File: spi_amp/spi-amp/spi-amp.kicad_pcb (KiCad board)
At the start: 4 copper layers, 26.9 x 54.8 mm, 25 parts, among them J1 IN+, J2 IN-, J3 OUT+, J4 OUT-, J5 Conn_01x06, U1 LMH6401, U2 LM78M05_TO220

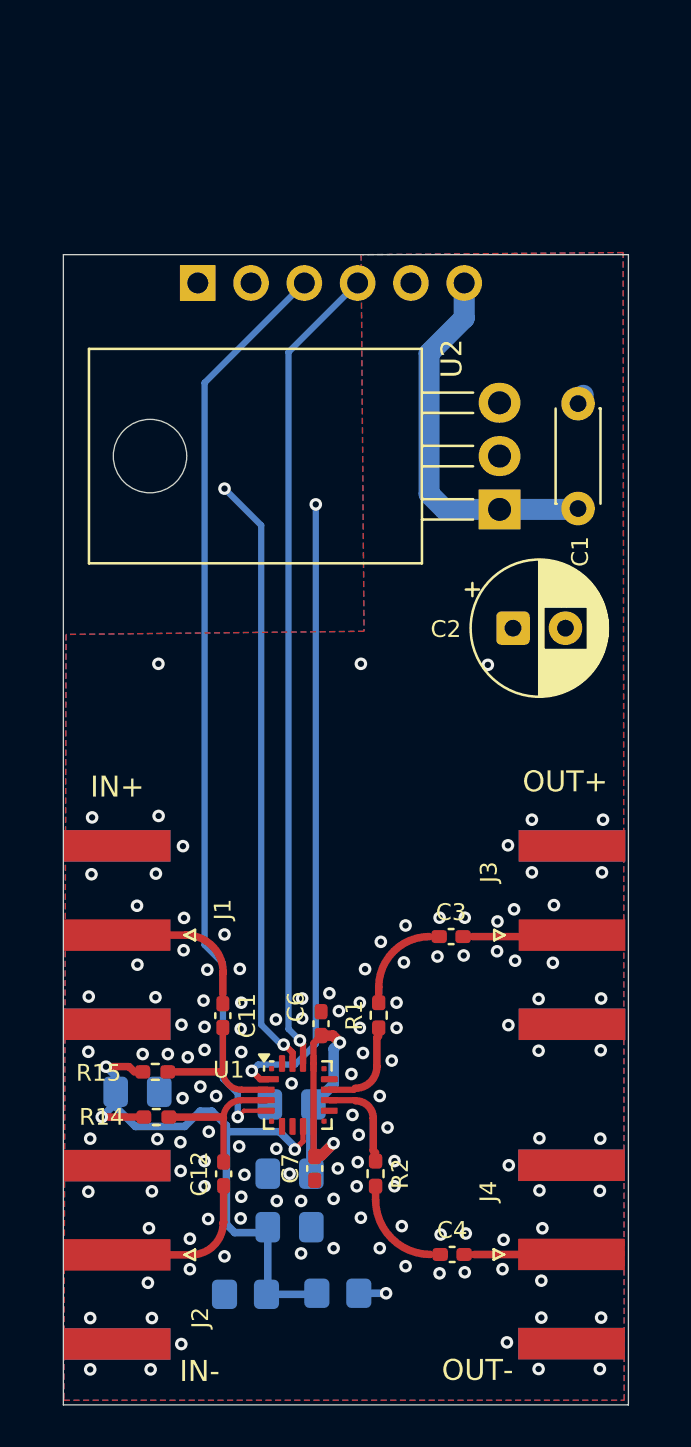
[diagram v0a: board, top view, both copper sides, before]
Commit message: ADCIO PCB done.
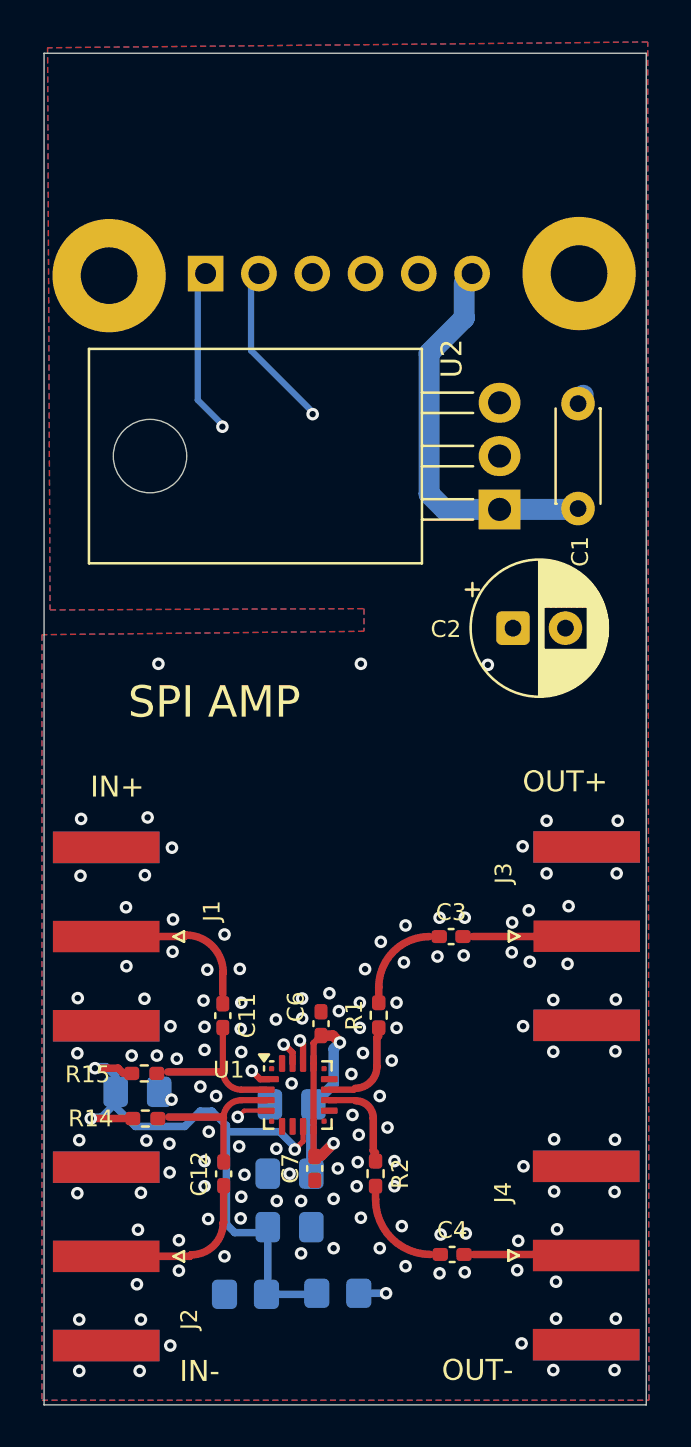
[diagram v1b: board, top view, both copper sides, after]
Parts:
- added H1: MountingHole_Pad, MountingHole:MountingHole_2.7mm_M2.5_Pad, F.Cu at (108.1, 52.9)
- added H2: MountingHole_Pad, MountingHole:MountingHole_2.7mm_M2.5_Pad, F.Cu at (130.5, 52.8)
- moved J3 0.70 mm to (130.9, 84.4)
- moved J4 0.70 mm to (130.8, 99.6)
- moved J5 0.59 mm to (112.7, 52.8)
- moved J1 0.53 mm to (108.0, 84.4)
- moved J2 0.53 mm to (108.0, 99.6)
- moved R14 0.53 mm to (109.8, 93.1)
- moved R15 0.53 mm to (109.8, 90.9)
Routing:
- net Net-(U1-Vocm): track 30.8 -> 31.9 mm
- net Net-(J2-In): track 7.64 -> 8.19 mm
- net Net-(J1-In): track 7.03 -> 7.58 mm
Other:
- board size 26.9 x 54.8 mm -> 28.7 x 64.4 mm
- board text added: "SPI AMP"
